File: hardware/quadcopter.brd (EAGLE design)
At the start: 116.6 x 116.8 mm, 96 parts, among them J1 AVR_SPI_PRG_6NS, J2 HEADER-0.1IN-2POS-MALE, J3 FTDI_BASICPTH, J5 HEADER-4POS-0.1IN-FEMALE, Q1 MOSFET-VISHAY-SOT23-N-MOSFET, Q2 MOSFET-VISHAY-SOT23-N-MOSFET, Q3 MOSFET-VISHAY-SOT23-N-MOSFET, Q4 MOSFET-VISHAY-SOT23-N-MOSFET, Q5 MOSFET-VISHAY-SOT23-N-MOSFET, U1 ATMEGA128RFA1, U2 IMU_LSM-ST-LSM9DS1-IMU-LGA, U3 MOTOR_PADS-MOLEX-0530470210, U4 MOTOR_PADS-MOLEX-0530470210, U5 MOTOR_PADS-MOLEX-0530470210, U6 MOTOR_PADS-MOLEX-0530470210, U7 3.3V, U8 NET_BRIDGE-BRIDGE-SMD, Y1 CRYSTAL5X3

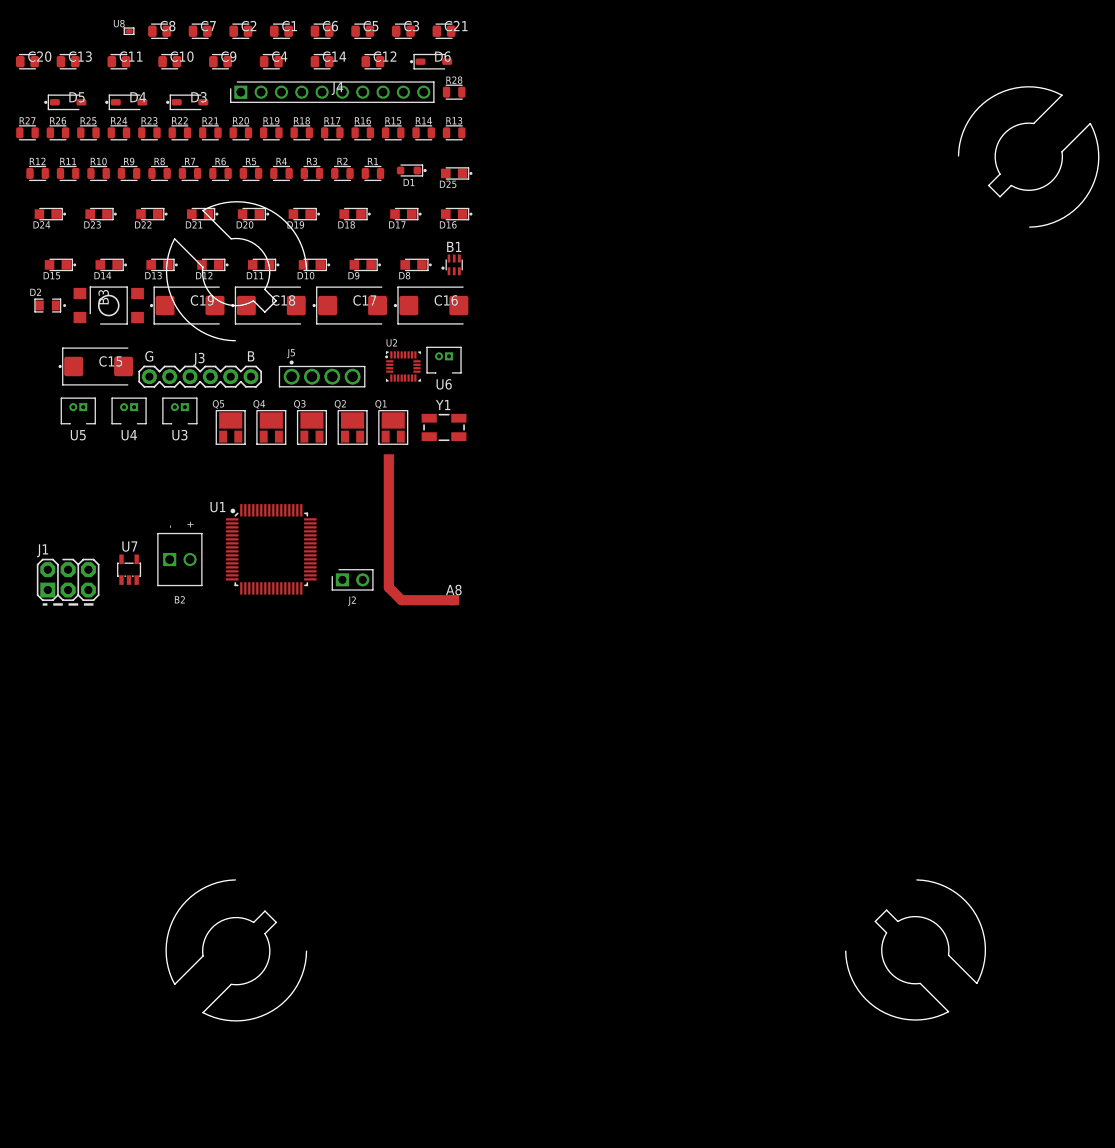
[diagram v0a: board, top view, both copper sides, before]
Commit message: Add files via upload
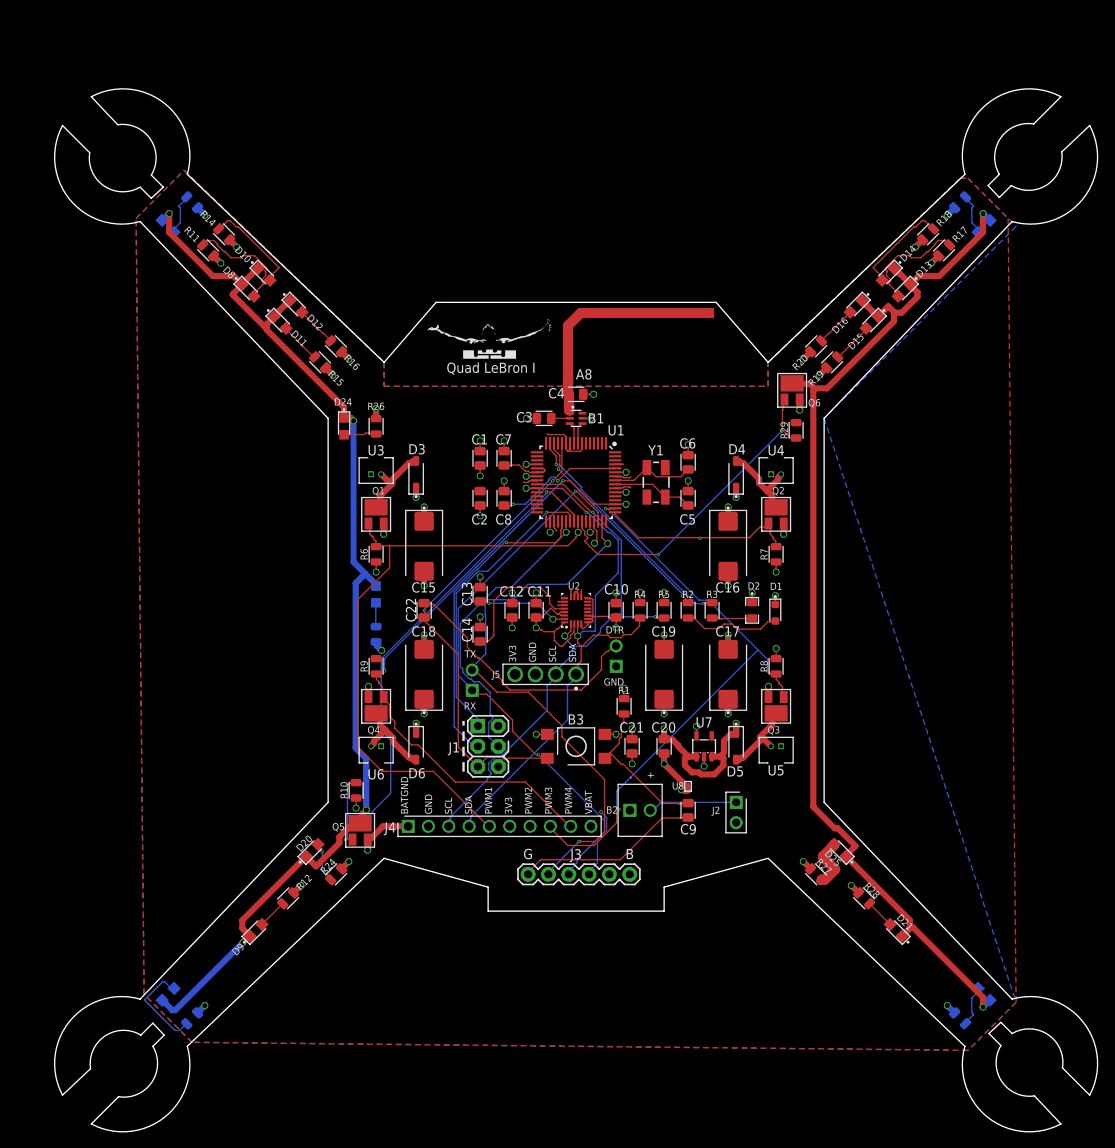
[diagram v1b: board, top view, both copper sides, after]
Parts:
- added C22: 0.1uF, quadparts_prebuilt:CAPC2012X140_HS
- added J6, J7: HEADER-0.1IN-2POS-FEMALE, quadparts_prebuilt:HDRV2W63P254_2X1_508X254H838_HS
- added Q6: MOSFET-VISHAY-SOT23-N-MOSFET, custom:SOT-23_N_MOSFET
- added R29: 10K, quadparts_prebuilt:RESC2012X60_HS
- added U$1: (no value), Logos:LEBRON_JAMES
- moved R25 155.3 mm to (48.0, -51.0), flipped to the bottom, turned to 45 degrees
- moved D23 147.5 mm to (51.0, -48.0), flipped to the bottom, turned to 225 degrees
- moved R27 135.3 mm to (30.0, -33.0), turned to 135 degrees
- moved D21 124.8 mm to (40.0, -40.0), turned to 315 degrees
- moved U8 117.4 mm to (14.0, -22.0), turned to 90 degrees
- moved C20 116.9 mm to (11.0, -17.0), turned to 90 degrees
- moved D5 116.0 mm to (20.0, -17.0), turned to 270 degrees
- moved R13 115.4 mm to (-48.0, -51.0), flipped to the bottom, turned to 135 degrees
- moved R28 113.0 mm to (36.0, -36.0), turned to 135 degrees
- moved C9 110.3 mm to (14.0, -25.0), turned to 90 degrees
- moved D15 102.0 mm to (37.0, 36.0), turned to 45 degrees
- moved R8 98.7 mm to (25.0, -7.00), turned to 270 degrees
- moved R22 97.9 mm to (48.0, 51.0), flipped to the bottom, turned to 315 degrees
- moved D22 97.6 mm to (-51.0, -48.0), flipped to the bottom, turned to 315 degrees
- moved D14 97.4 mm to (39.0, 42.0), turned to 45 degrees
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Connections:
- new net 34: Q6.G, R29.2, U1.42
- new net N$19: C22.1, J6.2
- new net N$39: D13.C, D14.C, D15.C, D16.C, D18.C, D21.C, D23.C, D25.C, Q6.D
- net BAT_GND: now also Q6.S
- net GND: now also J6.1, R29.1
- net N$38: no longer D13.C, D14.C, D15.C, D16.C, D18.C, D21.C, D23.C, D25.C
- net RESET: now also C22.2
- net RX0: now also J7.1
- net TX0: now also J7.2
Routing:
- net N$38: track 0.00 -> 140.6 mm, vias 0 -> 4
- net N$39: track 0.00 -> 137.6 mm, vias 0 -> 2
- net RESET: track 0.00 -> 79.8 mm, vias 0 -> 2
- net 3: track 0.00 -> 78.6 mm, vias 0 -> 1
- net 8: track 0.00 -> 78.4 mm, vias 0 -> 1
- net 5: track 0.00 -> 78.2 mm, vias 0 -> 3
- net 4: track 0.00 -> 74.9 mm, vias 0 -> 3
- net SDA: track 0.00 -> 70.2 mm, vias 0 -> 3
- net TX0: track 0.00 -> 69.6 mm, vias 0 -> 2
- net SCL: track 0.00 -> 69.5 mm, vias 0 -> 3
- net RX0: track 0.00 -> 69.4 mm, vias 0 -> 2
- net 9: track 0.00 -> 67.7 mm, vias 0 -> 3
- net GND: track 0.00 -> 57.5 mm, vias 0 -> 26
- net VBAT: track 0.00 -> 57.4 mm, vias 0 -> 27
- net 3V3: track 0.00 -> 56.2 mm, vias 0 -> 17
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- added copper zone on layer 15, net 3V3
- added copper zone on layer 2, net BAT_GND
- added copper zone on layer 1, net GND
- added copper zone on layer 16, net GND
- added copper zone on layer 2, net GND
- added copper zone on layer 15, net VBAT
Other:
- board size 116.6 x 116.8 mm -> 130.4 x 130.4 mm
- board text added: "3V3"
- board text added: "BATGND"
- board text added: "DTR"
- board text added: "GND"
- board text added: "PWM1"
- board text added: "PWM2"
- board text added: "PWM3"
- board text added: "PWM4"
- board text added: "RX"
- board text added: "SCL"
- board text added: "SDA"
- board text added: "TX"
- board text added: "VBAT"
